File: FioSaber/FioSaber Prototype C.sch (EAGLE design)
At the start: 20 parts, among them P1 WIICHUCK, T1 2N2222

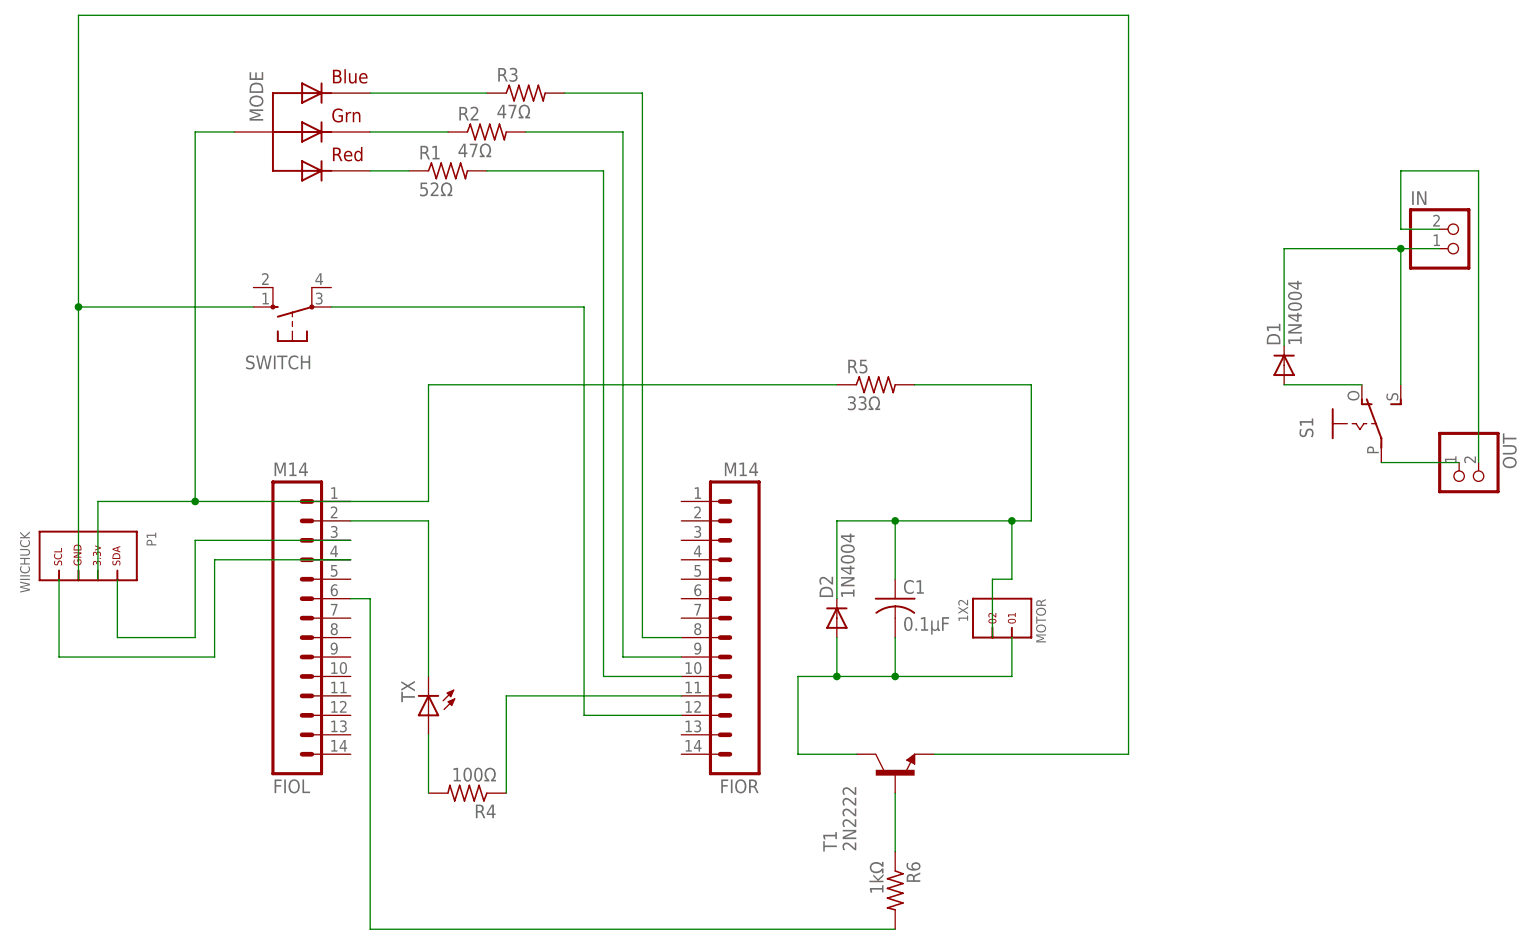
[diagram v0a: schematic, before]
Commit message: FioSaber Prototype C4
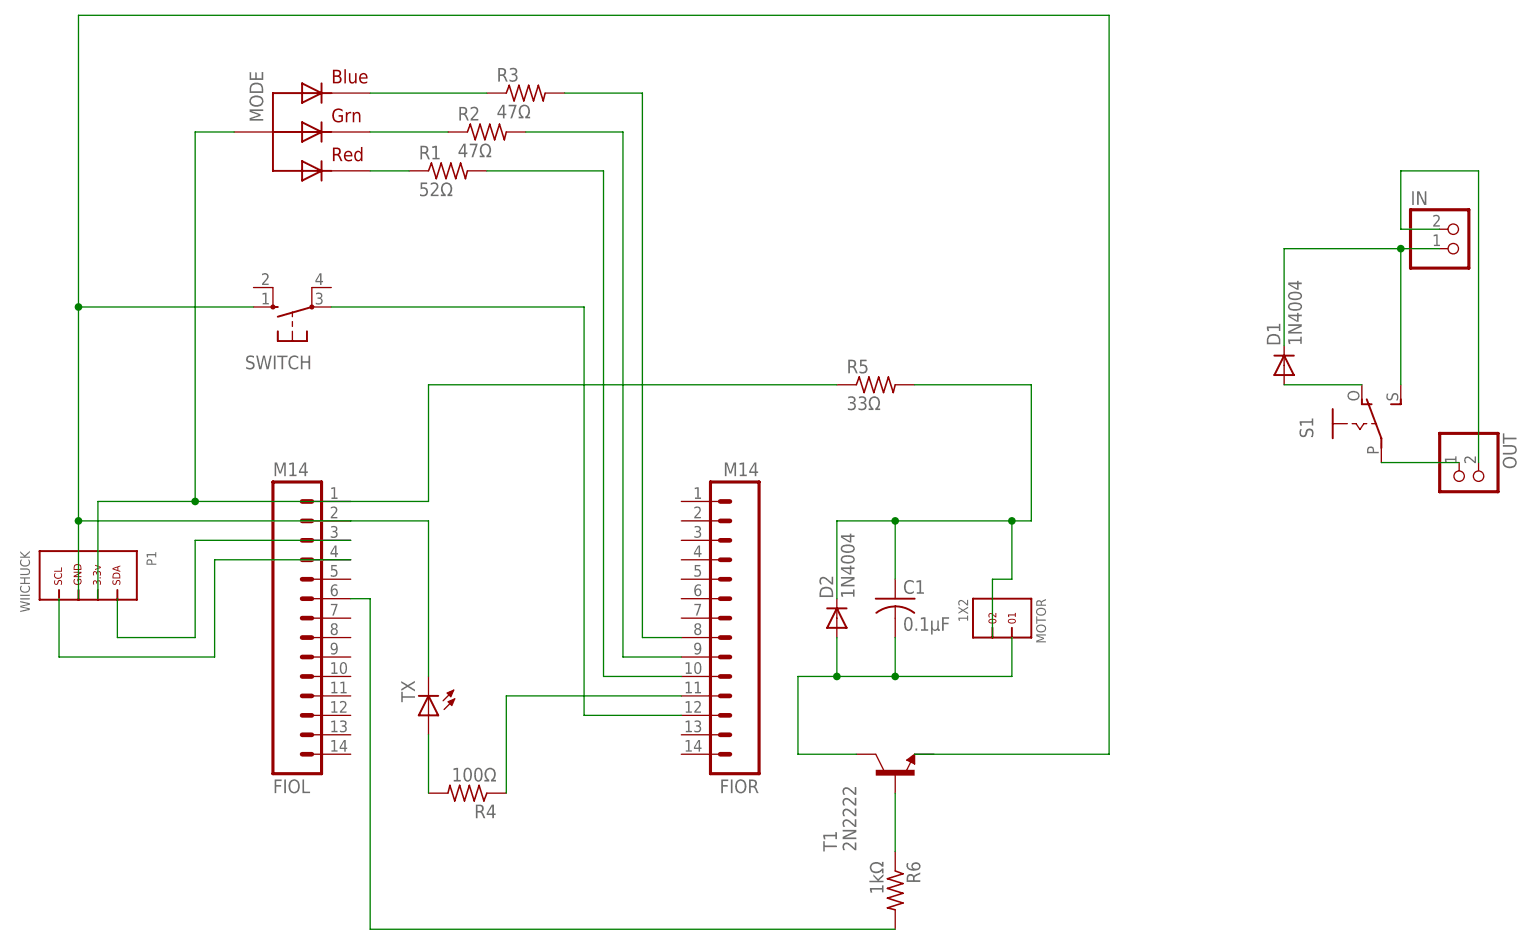
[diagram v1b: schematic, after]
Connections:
- removed net N$7: P1.SCL, SWITCH.S, T1.E
- net N$24: now also P1.SCL, SWITCH.S
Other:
- moved on the sheet: P1
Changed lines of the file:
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@@
 <instance part="FIOL" gate="G$1" x="48.26" y="91.44" rot="MR180"/>
 <instance part="FIOR" gate="G$1" x="111.76" y="91.44" rot="R180"/>
-<instance part="P1" gate="G$1" x="22.86" y="101.6" rot="R270"/>
+<instance part="P1" gate="G$1" x="22.86" y="99.06" rot="R270"/>
 <instance part="T1" gate="G$1" x="129.54" y="73.66" rot="R90"/>
 <instance part="C1" gate="G$1" x="129.54" y="96.52"/>
@@
 <pinref part="P1" gate="G$1" pin="SDA"/>
 <wire x1="38.1" y1="109.22" x2="25.4" y2="109.22" width="0.1524" layer="91"/>
-<wire x1="25.4" y1="109.22" x2="25.4" y2="99.06" width="0.1524" layer="91"/>
+<wire x1="25.4" y1="109.22" x2="25.4" y2="96.52" width="0.1524" layer="91"/>
 <junction x="38.1" y="109.22"/>
 <wire x1="38.1" y1="109.22" x2="38.1" y2="157.48" width="0.1524" layer="91"/>
@@
 </segment>
 </net>
-<net name="N$7" class="0">
-<segment>
-<pinref part="SWITCH" gate="1" pin="S"/>
-<pinref part="T1" gate="G$1" pin="E"/>
-<wire x1="22.86" y1="134.62" x2="22.86" y2="172.72" width="0.1524" layer="91"/>
-<wire x1="134.62" y1="76.2" x2="160.02" y2="76.2" width="0.1524" layer="91"/>
-<wire x1="160.02" y1="76.2" x2="160.02" y2="172.72" width="0.1524" layer="91"/>
-<wire x1="160.02" y1="172.72" x2="22.86" y2="172.72" width="0.1524" layer="91"/>
-<wire x1="45.72" y1="134.62" x2="22.86" y2="134.62" width="0.1524" layer="91"/>
-<junction x="22.86" y="134.62"/>
-<pinref part="P1" gate="G$1" pin="SCL"/>
-<wire x1="22.86" y1="134.62" x2="22.86" y2="99.06" width="0.1524" layer="91"/>
-</segment>
-</net>
 <net name="N$6" class="0">
 <segment>
@@
 <wire x1="40.64" y1="88.9" x2="20.32" y2="88.9" width="0.1524" layer="91"/>
 <pinref part="P1" gate="G$1" pin="GND"/>
-<wire x1="20.32" y1="88.9" x2="20.32" y2="99.06" width="0.1524" layer="91"/>
+<wire x1="20.32" y1="88.9" x2="20.32" y2="96.52" width="0.1524" layer="91"/>
 </segment>
 </net>
@@
 <segment>
 <pinref part="P1" gate="G$1" pin="PWR"/>
-<wire x1="27.94" y1="99.06" x2="27.94" y2="91.44" width="0.1524" layer="91"/>
+<wire x1="27.94" y1="96.52" x2="27.94" y2="91.44" width="0.1524" layer="91"/>
 <wire x1="27.94" y1="91.44" x2="38.1" y2="91.44" width="0.1524" layer="91"/>
 <wire x1="38.1" y1="91.44" x2="38.1" y2="104.14" width="0.1524" layer="91"/>
@@
 <pinref part="TX" gate="G$1" pin="C"/>
 <wire x1="68.58" y1="86.36" x2="68.58" y2="106.68" width="0.1524" layer="91"/>
-</segment>
-</net>
+<pinref part="P1" gate="G$1" pin="SCL"/>
+<wire x1="58.42" y1="106.68" x2="22.86" y2="106.68" width="0.1524" layer="91"/>
+<wire x1="22.86" y1="106.68" x2="22.86" y2="96.52" width="0.1524" layer="91"/>
+<wire x1="132.08" y1="76.2" x2="157.48" y2="76.2" width="0.1524" layer="91"/>
+<wire x1="157.48" y1="76.2" x2="157.48" y2="172.72" width="0.1524" layer="91"/>
+<wire x1="157.48" y1="172.72" x2="22.86" y2="172.72" width="0.1524" layer="91"/>
+<wire x1="22.86" y1="172.72" x2="22.86" y2="134.62" width="0.1524" layer="91"/>
+<junction x="22.86" y="106.68"/>
+<pinref part="SWITCH" gate="1" pin="S"/>
+<wire x1="22.86" y1="134.62" x2="22.86" y2="106.68" width="0.1524" layer="91"/>
+<wire x1="45.72" y1="134.62" x2="22.86" y2="134.62" width="0.1524" layer="91"/>
+<junction x="22.86" y="134.62"/>
+</segment>
+</net>
